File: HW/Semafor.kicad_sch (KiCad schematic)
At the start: 66 parts, among them J1 USB_C_Receptacle_USB2.0, J3 Conn_01x03_Male, M1 Motor_DC, Q2 Q_PMOS_GSD, Q3 Q_NMOS_GSD, Q4 Q_NMOS_GSD, Q5 Q_Photo_NPN, SW6 SW_SPDT, U1 ESP32-C3, U2 CN3058E, U3 LT1930, U4 E22-900T22D, U5 AT42QT1070-S

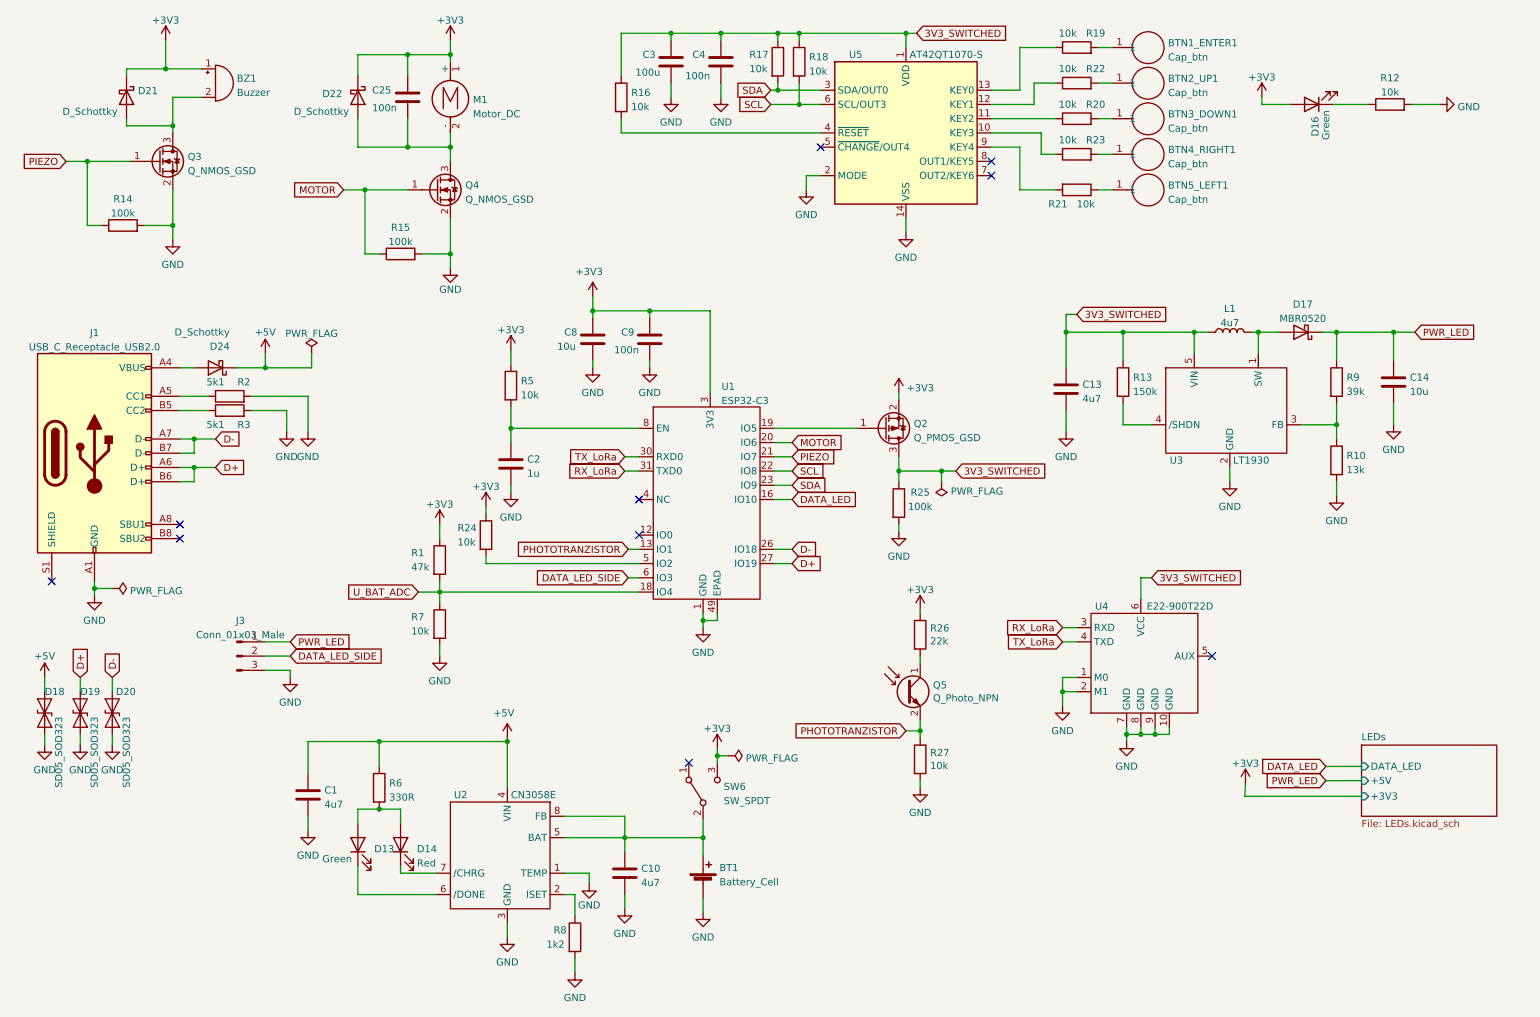
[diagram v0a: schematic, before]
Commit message: continue routing
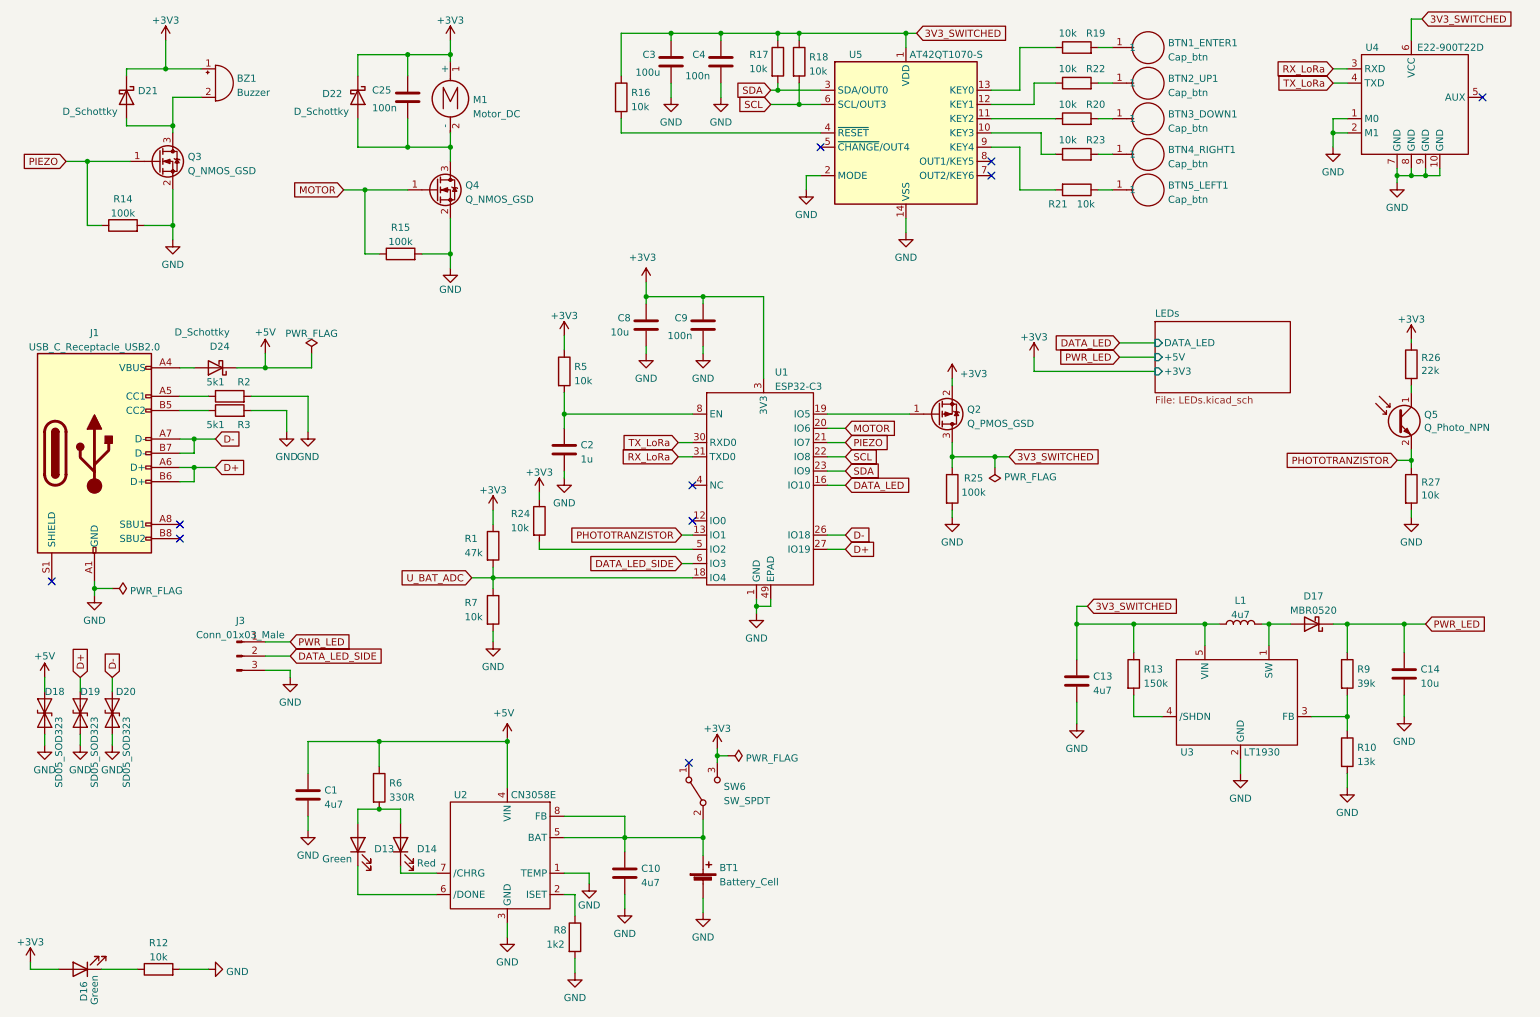
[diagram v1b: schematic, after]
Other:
- moved on the sheet: C13, C14, C2, C8, C9, D16, D17, L1, Q2, Q5, R1, R10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
